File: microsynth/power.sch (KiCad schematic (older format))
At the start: 10 parts, among them J2 Conn_01x03_Male, J3 Conn_01x06_Male, J4 Conn_01x04_Male

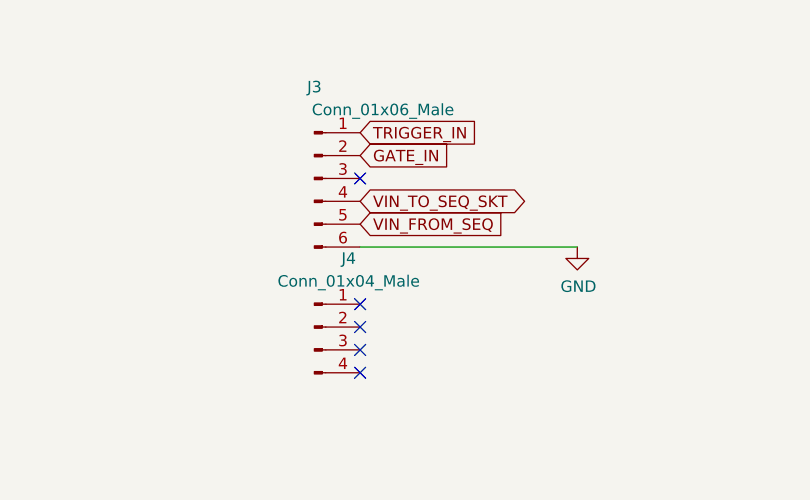
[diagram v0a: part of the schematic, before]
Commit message: Clean up and reroute
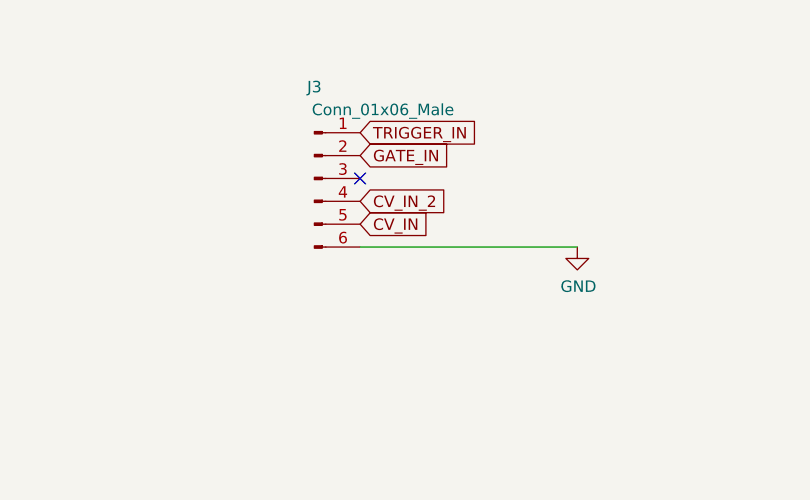
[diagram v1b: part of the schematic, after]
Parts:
- removed J4: Conn_01x04_Male, Connector_PinHeader_2.54mm:PinHeader_1x04_P2.54mm_Vertical, symbol Connector:Conn_01x04_Male
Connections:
- net VIN_FROM_SEQ renamed CV_IN
- net VIN_TO_SEQ_SKT renamed CV_IN_2
- no-connect marks 5 -> 1
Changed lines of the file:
@@
 Text GLabel 5900 2600 2    50   Input ~ 0
 TRIGGER_IN
-Text GLabel 5900 2900 2    50   BiDi ~ 0
-VIN_TO_SEQ_SKT
+Text GLabel 5900 3000 2    50   Input ~ 0
+CV_IN
 $Comp
 L Connector:Conn_01x03_Male J2
@@
 F 3 "~" H 6500 1400 50  0001 C CNN
 	1    6500 1400
-	1    0    0    -1
-$EndComp
-$Comp
-L Connector:Conn_01x04_Male J4
-U 1 1 5F1FE242
-P 5700 3450
-F 0 "J4" H 5850 3750 50  0000 C CNN
-F 1 "Conn_01x04_Male" H 5850 3650 50  0000 C CNN
-F 2 "Connector_PinHeader_2.54mm:PinHeader_1x04_P2.54mm_Vertical" H 5700 3450 50  0001 C CNN
-F 3 "~" H 5700 3450 50  0001 C CNN
-	1    5700 3450
 	1    0    0    -1
 $EndComp
@@
 Wire Wire Line
 	7050 1300 6700 1300
-Text GLabel 5900 3000 2    50   Input ~ 0
-VIN_FROM_SEQ
+Text GLabel 5900 2900 2    50   Input ~ 0
+CV_IN_2
 $Comp
 L Mechanical:MountingHole H1
@@
 	7750 1500 7450 1500
 Connection ~ 7450 1500
-NoConn ~ 5900 3350
-NoConn ~ 5900 3450
-NoConn ~ 5900 3550
-NoConn ~ 5900 3650
 NoConn ~ 5900 2800
 Text GLabel 5900 2700 2    50   Input ~ 0
